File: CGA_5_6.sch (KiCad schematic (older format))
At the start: 8 parts, among them U13 74LS08, U14 74LS32, U15 74LS00, U20 74LS04, U21 74LS174, U42 74LS86, U43 74S74, U64 74LS164

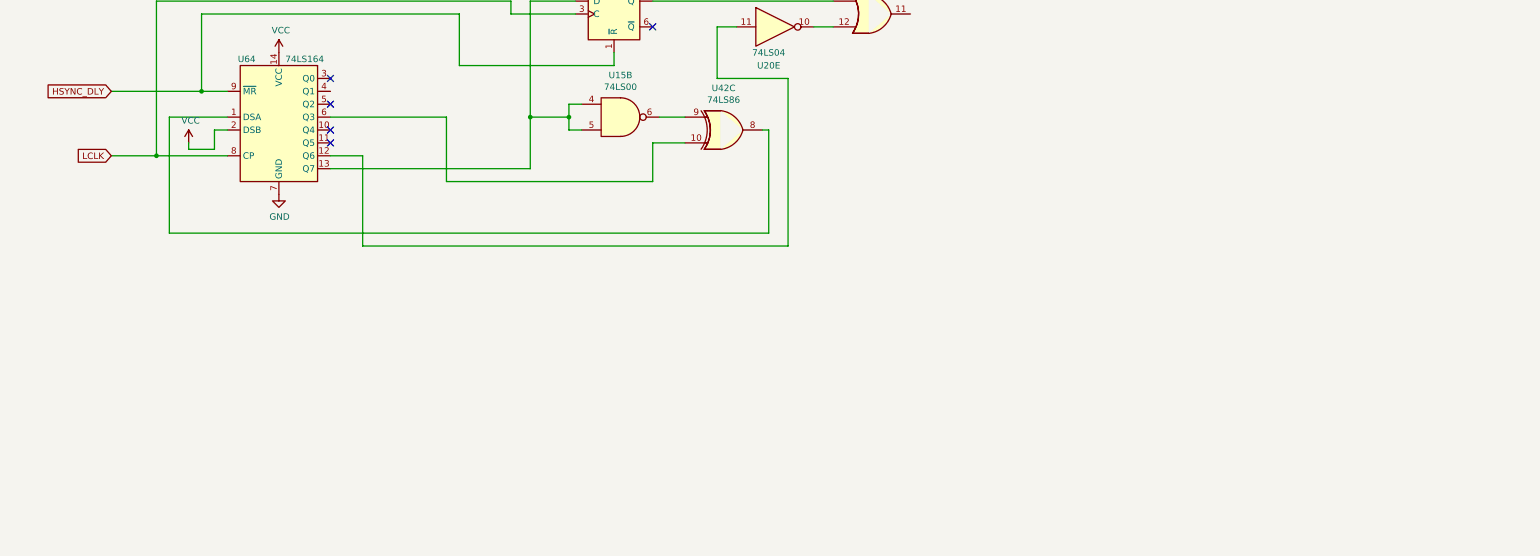
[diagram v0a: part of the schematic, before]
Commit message: More sheet 5
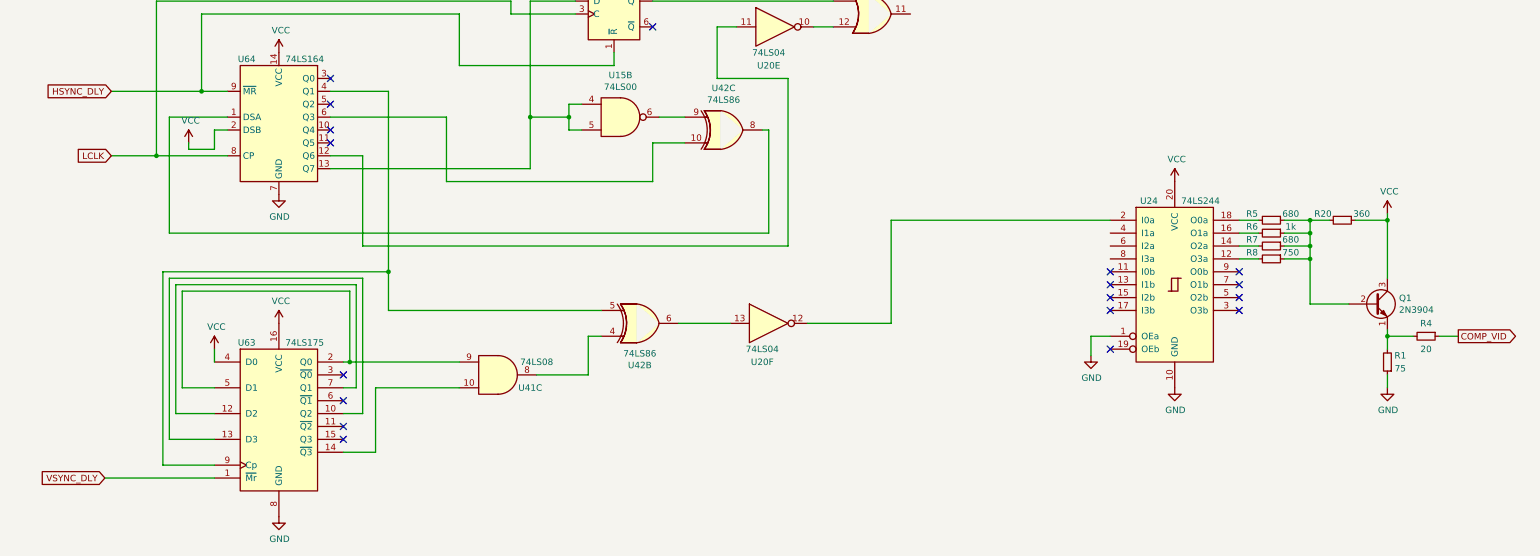
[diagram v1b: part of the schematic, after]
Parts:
- added Q1: 2N3904, Package_TO_SOT_THT:TO-92_Inline, symbol Transistor_BJT:2N3904
- added R1: 75, Resistor_THT:R_Axial_DIN0207_L6.3mm_D2.5mm_P10.16mm_Horizontal, symbol Device:R_Small
- added R20: 360, Resistor_THT:R_Axial_DIN0207_L6.3mm_D2.5mm_P10.16mm_Horizontal, symbol Device:R_Small
- added R4: 20, Resistor_THT:R_Axial_DIN0207_L6.3mm_D2.5mm_P10.16mm_Horizontal, symbol Device:R_Small
- added R5, R7: 680, Resistor_THT:R_Axial_DIN0207_L6.3mm_D2.5mm_P10.16mm_Horizontal, symbol Device:R_Small
- added R6: 1k, Resistor_THT:R_Axial_DIN0207_L6.3mm_D2.5mm_P10.16mm_Horizontal, symbol Device:R_Small
- added R8: 750, Resistor_THT:R_Axial_DIN0207_L6.3mm_D2.5mm_P10.16mm_Horizontal, symbol Device:R_Small
- added unit 6 of U20
- added U24: 74LS244, Package_DIP:DIP-20_W7.62mm_LongPads, symbol 74xx:74LS244
- added U41: 74LS08, Package_DIP:DIP-14_W7.62mm_LongPads, symbol 74xx:74LS08
- added unit 2 of U42
- added U63: 74LS175, Package_DIP:DIP-16_W7.62mm_LongPads, symbol 74xx:74LS175
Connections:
- net GND: now also R1.1, U24.1 (OEa), U24.10 (GND), U63.8 (GND)
- net VCC: now also Q1.3 (C), R20.1, U24.20 (VCC), U63.16 (VCC), U63.4 (D0)
- net VSYNC_DLY: now also U63.1 (~Mr)
- net at U64.4 (Q1): now also U42.5, U63.9 (Cp)
- new net: U63.10 (Q2), U63.13 (D3)
- new net: U63.12 (D2), U63.7 (Q1)
- new net: U41.10, U63.14 (~Q3)
- new net: U41.9, U63.2 (Q0), U63.5 (D1)
- new net: U41.8, U42.4
- new net: U20.13, U42.6
- new net: U20.12, U24.2 (I0a)
- new net: R8.2, U24.12 (O3a)
- new net: R7.2, U24.14 (O2a)
- new net: R6.2, U24.16 (O1a)
- new net: R5.2, U24.18 (O0a)
- new net: Q1.2 (B), R20.2, R5.1, R6.1, R7.1, R8.1
- new net: Q1.1 (E), R1.2, R4.2
- new net COMP_VID: R4.1
- no-connect marks 5 -> 18

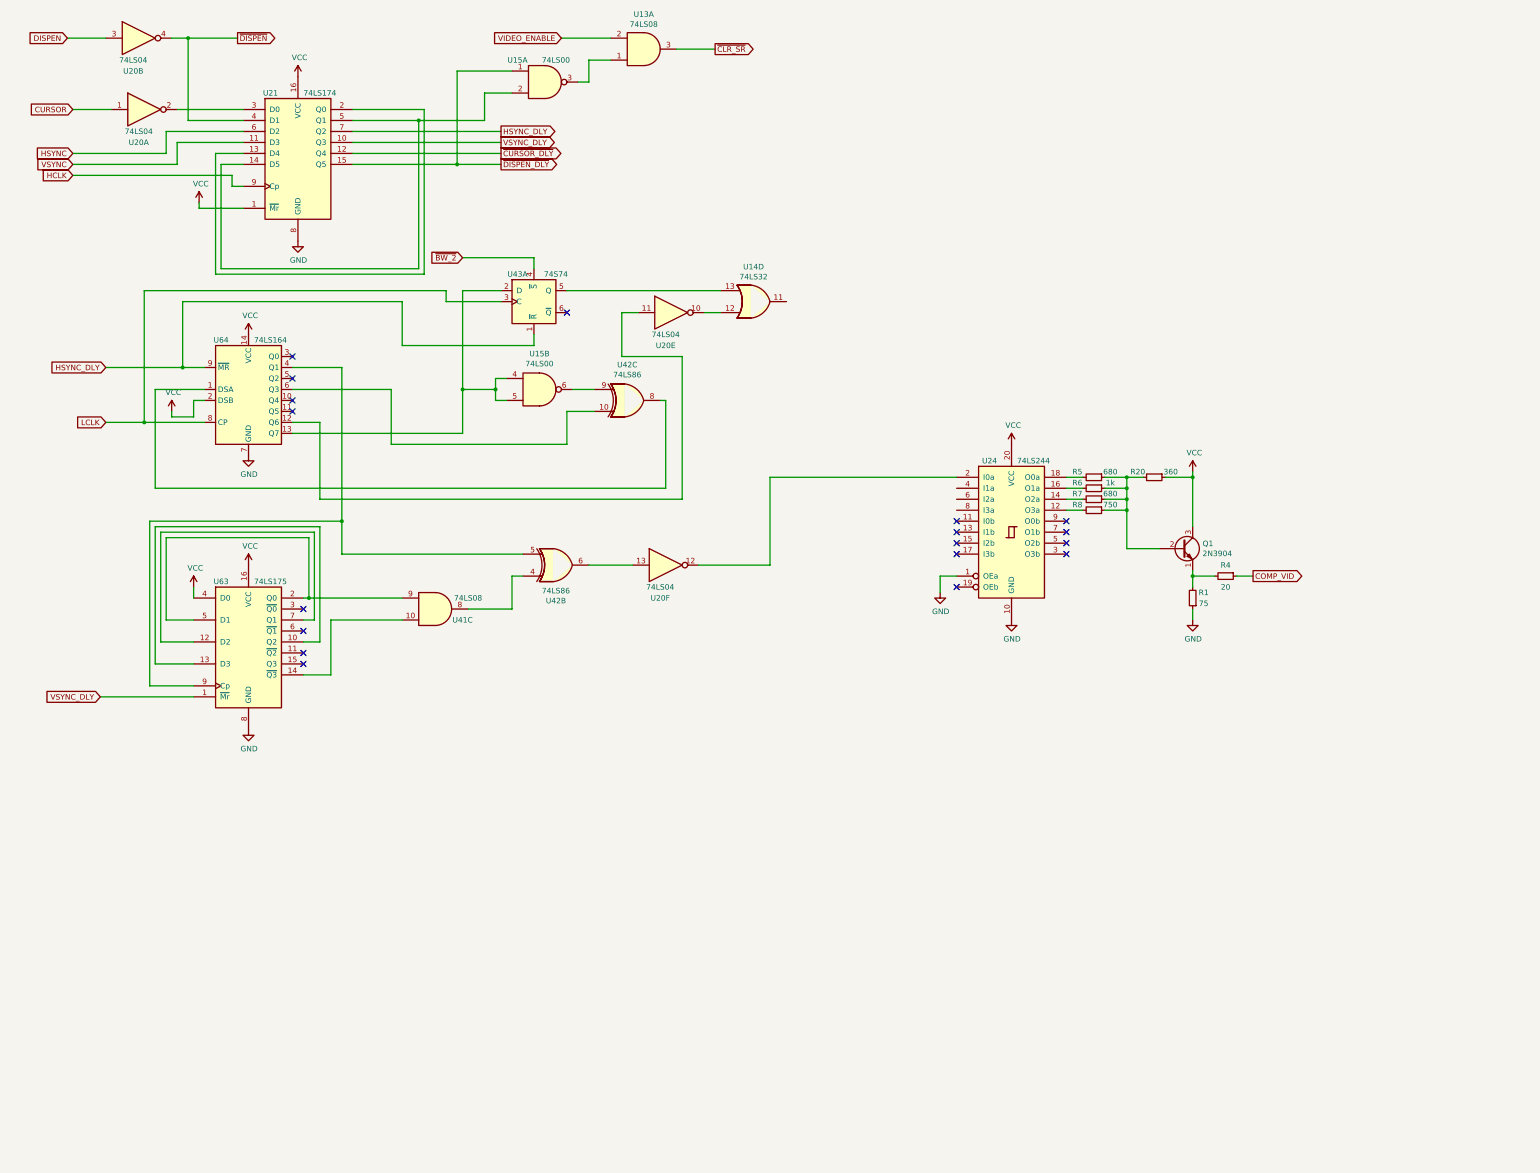
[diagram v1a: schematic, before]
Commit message: More sheet 5
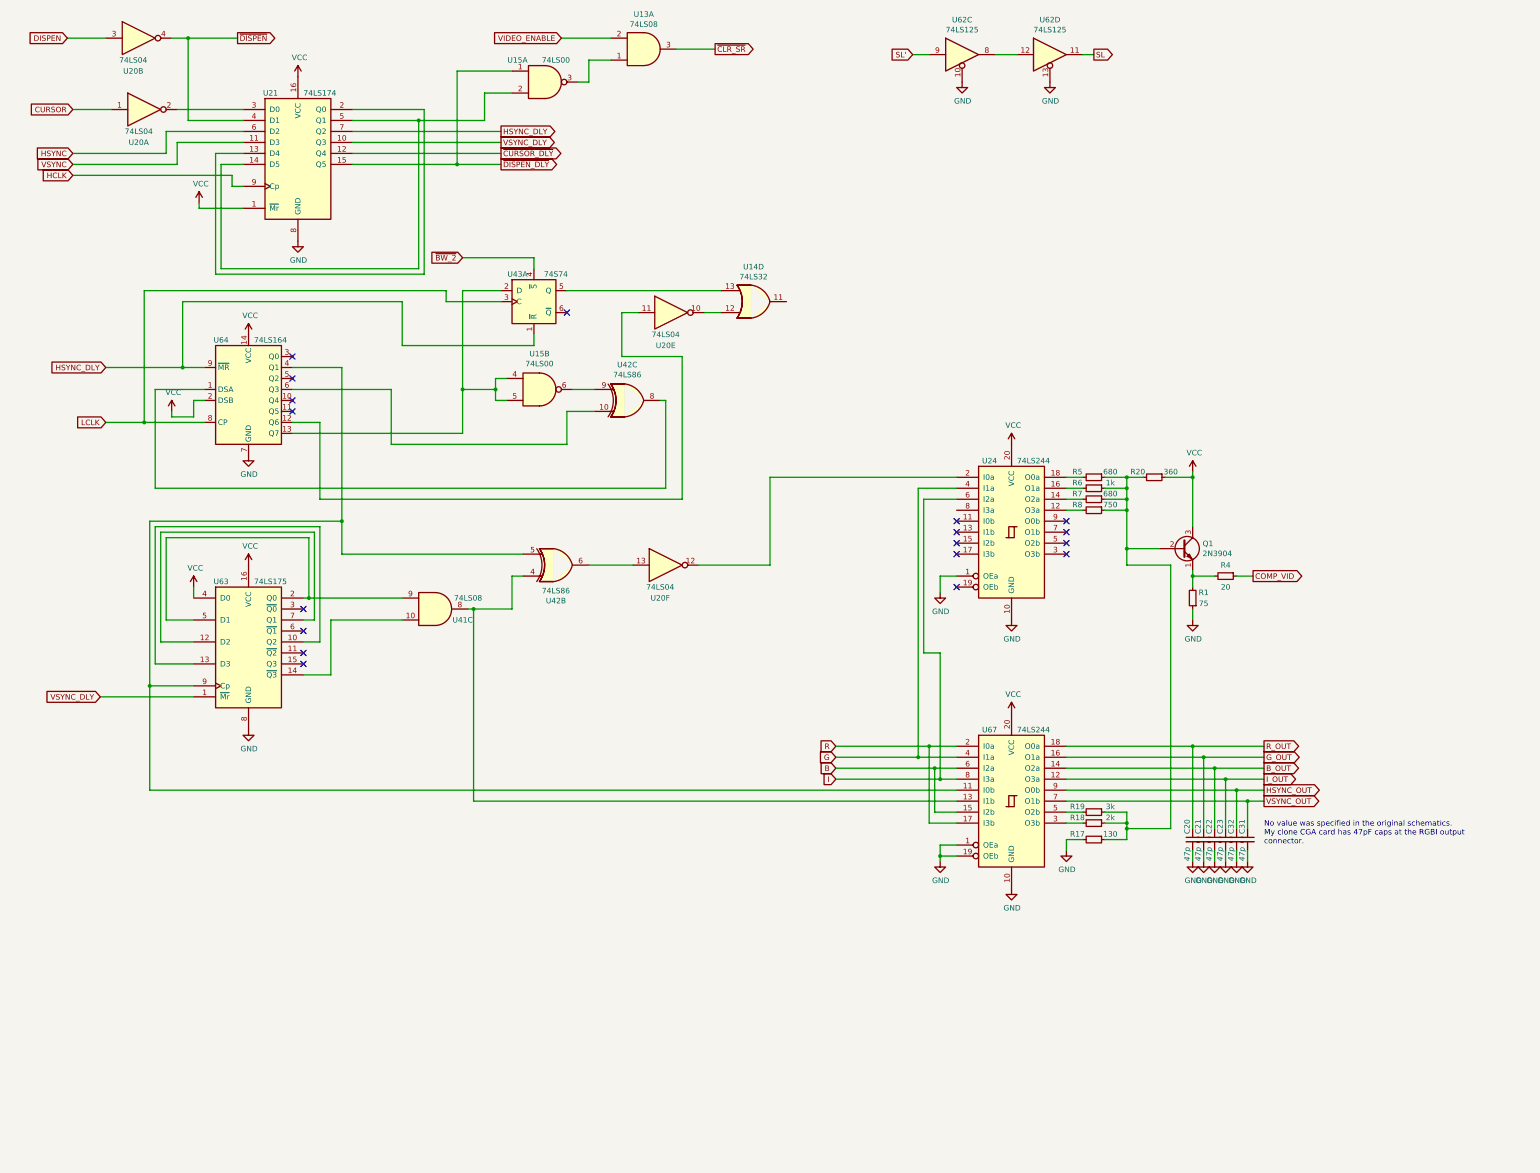
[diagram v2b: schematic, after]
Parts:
- added C20, C21, C22, C23, C31, C32: 47p, Capacitor_THT:C_Disc_D4.3mm_W1.9mm_P5.00mm, symbol Device:C_Small
- added R17: 130, Resistor_THT:R_Axial_DIN0207_L6.3mm_D2.5mm_P10.16mm_Horizontal, symbol Device:R_Small
- added R18: 2k, Resistor_THT:R_Axial_DIN0207_L6.3mm_D2.5mm_P10.16mm_Horizontal, symbol Device:R_Small
- added R19: 3k, Resistor_THT:R_Axial_DIN0207_L6.3mm_D2.5mm_P10.16mm_Horizontal, symbol Device:R_Small
- added U62: 74LS125, Package_DIP:DIP-14_W10.16mm_LongPads, symbol 74xx:74LS125
- added U67: 74LS244, Package_DIP:DIP-20_W7.62mm_LongPads, symbol 74xx:74LS244
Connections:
- net GND: now also C20.2, C21.2, C22.2, C23.2, C31.2, C32.2, R17.2, U62.10, U62.13, U67.1 (OEa), U67.10 (GND), U67.19 (OEb)
- net VCC: now also U67.20 (VCC)
- net at U42.5, U63.9 (Cp), U64.4 (Q1): now also U67.11 (I0b)
- net at U41.8, U42.4: now also U67.13 (I1b)
- net G: now reaches U24.4 (I1a)
- net G: now also U67.4 (I1a)
- net I: now reaches U24.6 (I2a)
- net I: now also U67.8 (I3a)
- net at Q1.2 (B), R20.2, R5.1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: now also R17.1, R18.1, R19.1
- new net: U62.12, U62.8
- new net: R18.2, U67.3 (O3b)
- new net: R19.2, U67.5 (O2b)
- new net B: U67.15 (I2b), U67.6 (I2a)
- new net B_OUT: C22.1, U67.14 (O2a)
- new net G_OUT: C21.1, U67.16 (O1a)
- new net HSYNC_OUT: C32.1, U67.9 (O0b)
- new net I_OUT: C23.1, U67.12 (O3a)
- new net R: U67.17 (I3b), U67.2 (I0a)
- new net R_OUT: C20.1, U67.18 (O0a)
- new net SL: U62.11
- new net SL': U62.9
- new net VSYNC_OUT: C31.1, U67.7 (O1b)
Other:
- note added: "No value was specified in the original schematics.\nMy clone CGA card has 47pF caps at the RGBI output\nconnector."
